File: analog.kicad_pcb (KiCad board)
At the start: 2 copper layers, 80 x 40 mm, 65 parts, among them P1 CONN_01X09, P2 CONN_01X06, P3 CONN_01X06, P4 CONN_01X05, U1 LM2940, U2 TLC2543

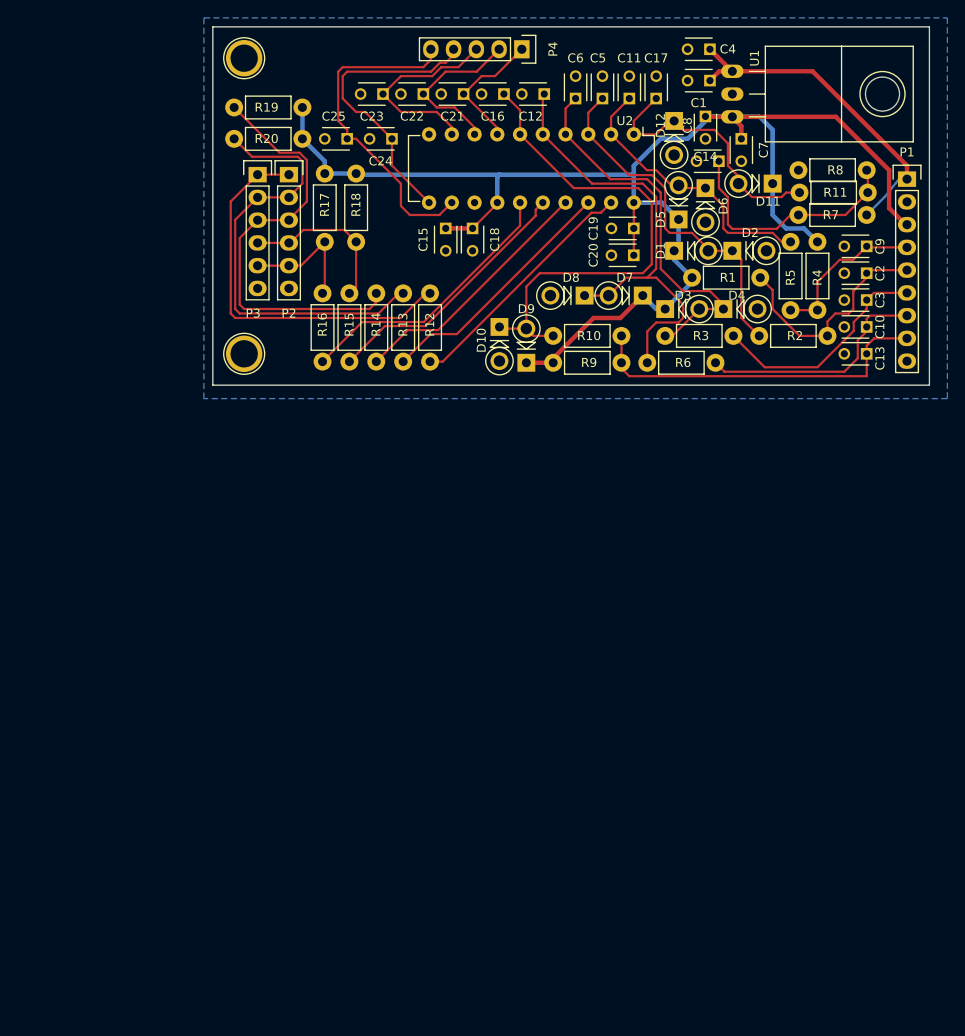
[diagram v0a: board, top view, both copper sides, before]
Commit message: fixups
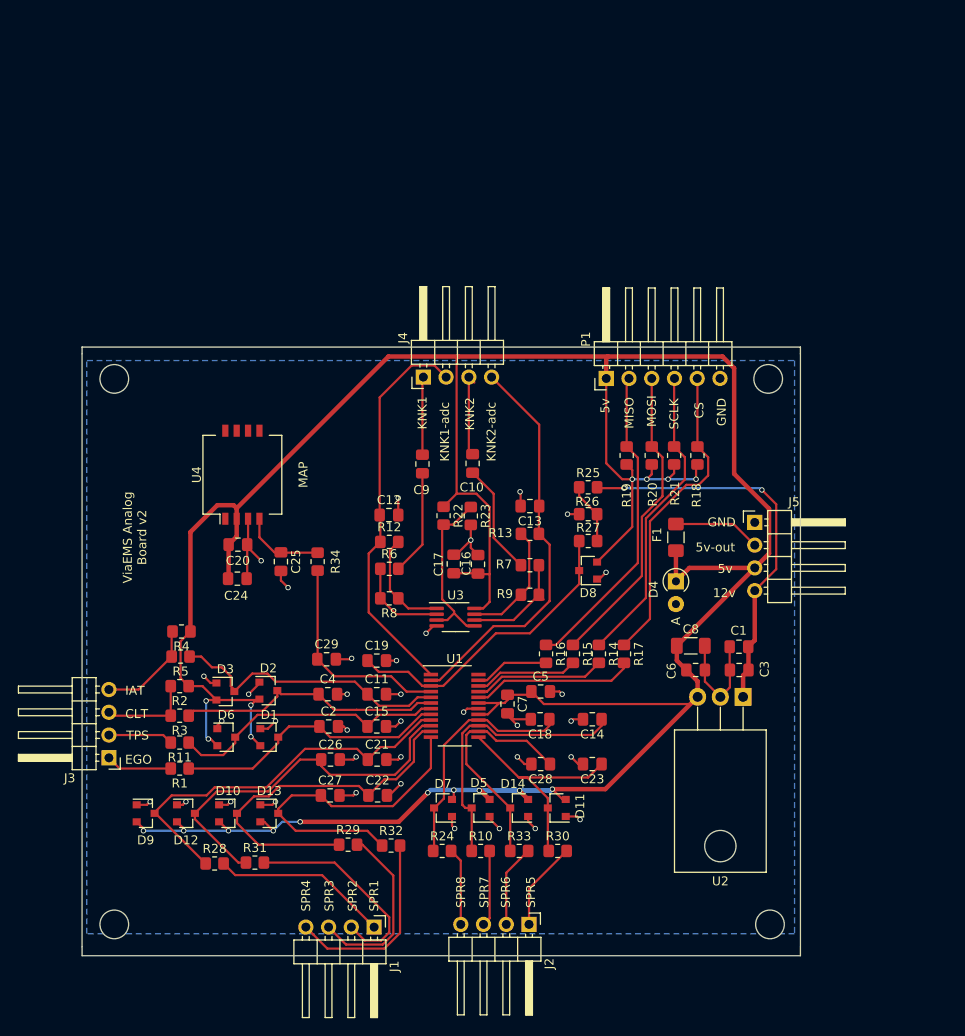
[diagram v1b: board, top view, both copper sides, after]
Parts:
- removed ?: 1pin, Connect:1pin
- removed P2, P3: CONN_01X06, Pin_Headers:Pin_Header_Straight_1x06
- removed P4: CONN_01X05, Pin_Headers:Pin_Header_Straight_1x05
- removed the REF** at (48.5, 69.0)
- added C26: 0.47 uF, Capacitor_SMD:C_0805_2012Metric_Pad1.18x1.45mm_HandSolder, F.Cu at (58.1, 147.3)
- added C27: 0.47 uF, Capacitor_SMD:C_0805_2012Metric_Pad1.18x1.45mm_HandSolder, F.Cu at (58.1, 151.3)
- added C28: 0.47 uF, Capacitor_SMD:C_0805_2012Metric_Pad1.18x1.45mm_HandSolder, F.Cu at (81.6, 147.8)
- added C29: 0.47 uF, Capacitor_SMD:C_0805_2012Metric_Pad1.18x1.45mm_HandSolder, F.Cu at (57.7, 136.1)
- added D13: BAT54S, Package_TO_SOT_SMD:SOT-23, F.Cu at (51.3, 153.3)
- added D14: BAT54S, Package_TO_SOT_SMD:SOT-23, F.Cu at (79.2, 152.7)
- added F1: 500 mA, Fuse:Fuse_1206_3216Metric_Pad1.42x1.75mm_HandSolder, F.Cu at (96.7, 122.5)
- added J1: SPARE1, Connector_PinHeader_2.54mm:PinHeader_1x04_P2.54mm_Horizontal, F.Cu at (63.0, 166.0)
- added J2: SPARE2, Connector_PinHeader_2.54mm:PinHeader_1x04_P2.54mm_Horizontal, F.Cu at (80.3, 165.7)
- added J3: MAIN, Connector_PinHeader_2.54mm:PinHeader_1x04_P2.54mm_Horizontal, F.Cu at (33.4, 147.1)
- added J4: KNOCK, Connector_PinHeader_2.54mm:PinHeader_1x04_P2.54mm_Horizontal, F.Cu at (68.5, 104.6)
- added J5: POWER, Connector_PinHeader_2.54mm:PinHeader_1x04_P2.54mm_Horizontal, F.Cu at (105.5, 120.8)
- added R21: 10k, Resistor_SMD:R_0805_2012Metric_Pad1.20x1.40mm_HandSolder, F.Cu at (96.5, 113.3)
- added R22: 1000, Resistor_SMD:R_0805_2012Metric_Pad1.20x1.40mm_HandSolder, F.Cu at (70.8, 120.1)
- added R23: 1000, Resistor_SMD:R_0805_2012Metric_Pad1.20x1.40mm_HandSolder, F.Cu at (73.8, 120.1)
- added R24: 220, Resistor_SMD:R_0805_2012Metric_Pad1.20x1.40mm_HandSolder, F.Cu at (70.6, 157.5)
- added R25: 3.9k, Resistor_SMD:R_0805_2012Metric_Pad1.20x1.40mm_HandSolder, F.Cu at (86.9, 116.9)
- added R26: 1k, Resistor_SMD:R_0805_2012Metric_Pad1.20x1.40mm_HandSolder, F.Cu at (86.9, 119.9)
- added R27: 220, Resistor_SMD:R_0805_2012Metric_Pad1.20x1.40mm_HandSolder, F.Cu at (86.9, 122.9)
- added R28: 220, Resistor_SMD:R_0805_2012Metric_Pad1.20x1.40mm_HandSolder, F.Cu at (45.2, 158.9)
- added R29: 220, Resistor_SMD:R_0805_2012Metric_Pad1.20x1.40mm_HandSolder, F.Cu at (60.1, 156.8)
- added R30: 220, Resistor_SMD:R_0805_2012Metric_Pad1.20x1.40mm_HandSolder, F.Cu at (83.5, 157.5)
- added R31: 220, Resistor_SMD:R_0805_2012Metric_Pad1.20x1.40mm_HandSolder, F.Cu at (49.7, 158.8)
- added R32: 220, Resistor_SMD:R_0805_2012Metric_Pad1.20x1.40mm_HandSolder, F.Cu at (64.9, 156.9)
- added R33: 220, Resistor_SMD:R_0805_2012Metric_Pad1.20x1.40mm_HandSolder, F.Cu at (79.2, 157.5)
- added R34: 220, Resistor_SMD:R_0805_2012Metric_Pad1.20x1.40mm_HandSolder, F.Cu at (56.7, 125.2)
- added REF**: MountingHole_3.2mm_M3, MountingHole:MountingHole_3.2mm_M3, F.Cu at (34.0, 165.7)
- added REF**: MountingHole_3.2mm_M3, MountingHole:MountingHole_3.2mm_M3, F.Cu at (107.2, 165.7)
- added REF**: MountingHole_3.2mm_M3, MountingHole:MountingHole_3.2mm_M3, F.Cu at (107.0, 104.8)
- added REF**: MountingHole_3.2mm_M3, MountingHole:MountingHole_3.2mm_M3, F.Cu at (34.0, 104.8)
- added U3: MCP6002-xSN, Package_SO:MSOP-8_3x3mm_P0.65mm, F.Cu at (72.1, 131.4)
- added U4: MPXA6400A, Sensor_Pressure:Freescale_98ARH99089A, F.Cu at (48.3, 115.5)
- C1, C10, C13, C21, C22, C23, C3, C7, C9: footprint Capacitors_ThroughHole:C_Disc_D3_P2.5 -> Capacitor_SMD:C_0805_2012Metric_Pad1.18x1.45mm_HandSolder
- C11, C16: value 0.47 uF -> 1 uF; footprint Capacitors_ThroughHole:C_Disc_D3_P2.5 -> Capacitor_SMD:C_0805_2012Metric_Pad1.18x1.45mm_HandSolder
- C12, C17, C25, C5, C6: value 0.47 uF -> 0.1 uF; footprint Capacitors_ThroughHole:C_Disc_D3_P2.5 -> Capacitor_SMD:C_0805_2012Metric_Pad1.18x1.45mm_HandSolder
- C14, C2: value 0.1 uF -> 0.47 uF; footprint Capacitors_ThroughHole:C_Disc_D3_P2.5 -> Capacitor_SMD:C_0805_2012Metric_Pad1.18x1.45mm_HandSolder
- C15, C19, C4: value 0.1 uF -> 1 uF; footprint Capacitors_ThroughHole:C_Disc_D3_P2.5 -> Capacitor_SMD:C_0805_2012Metric_Pad1.18x1.45mm_HandSolder
- C18: value 10 uF -> 0.47 uF; footprint Capacitors_ThroughHole:C_Disc_D3_P2.5 -> Capacitor_SMD:C_0805_2012Metric_Pad1.18x1.45mm_HandSolder
- C20: value 10 uF -> 0.01 uF; footprint Capacitors_ThroughHole:C_Disc_D3_P2.5 -> Capacitor_SMD:C_0805_2012Metric_Pad1.18x1.45mm_HandSolder
- C24: value 0.47 uF -> 0.33 uF; footprint Capacitors_ThroughHole:C_Disc_D3_P2.5 -> Capacitor_SMD:C_0805_2012Metric_Pad1.18x1.45mm_HandSolder
- C8: footprint Capacitors_ThroughHole:C_Disc_D3_P2.5 -> Capacitor_SMD:C_1206_3216Metric_Pad1.33x1.80mm_HandSolder
- D1, D10, D11, D12, D2, D3, D5, D6, D7, D8, D9: value 1N5818 -> BAT54S; footprint Diodes_ThroughHole:Diode_DO-41_SOD81_Vertical_KathodeUp -> Package_TO_SOT_SMD:SOT-23
- D4: value 1N5818 -> 5.4 V; footprint Diodes_ThroughHole:Diode_DO-41_SOD81_Vertical_KathodeUp -> Diode_THT:D_A-405_P2.54mm_Vertical_AnodeUp
- P1: value CONN_01X09 -> CONN_01X06; footprint Pin_Headers:Pin_Header_Straight_1x09 -> Connector_PinHeader_2.54mm:PinHeader_1x06_P2.54mm_Horizontal
- R1: value 2.49k -> 220; footprint Resistors_ThroughHole:Resistor_Horizontal_RM7mm -> Resistor_SMD:R_0805_2012Metric_Pad1.20x1.40mm_HandSolder
- R10, R11, R3, R5: value 470 -> 220; footprint Resistors_ThroughHole:Resistor_Horizontal_RM7mm -> Resistor_SMD:R_0805_2012Metric_Pad1.20x1.40mm_HandSolder
- R12, R13: value 100 -> 120; footprint Resistors_ThroughHole:Resistor_Horizontal_RM7mm -> Resistor_SMD:R_0805_2012Metric_Pad1.20x1.40mm_HandSolder
- R14, R15, R16, R18, R19, R20, R4: footprint Resistors_ThroughHole:Resistor_Horizontal_RM7mm -> Resistor_SMD:R_0805_2012Metric_Pad1.20x1.40mm_HandSolder
- R17: value 10k -> 100; footprint Resistors_ThroughHole:Resistor_Horizontal_RM7mm -> Resistor_SMD:R_0805_2012Metric_Pad1.20x1.40mm_HandSolder
- R2: value 470 -> 2.49k; footprint Resistors_ThroughHole:Resistor_Horizontal_RM7mm -> Resistor_SMD:R_0805_2012Metric_Pad1.20x1.40mm_HandSolder
- R6: value 470 -> 1000; footprint Resistors_ThroughHole:Resistor_Horizontal_RM7mm -> Resistor_SMD:R_0805_2012Metric_Pad1.20x1.40mm_HandSolder
- R7: value 3.9k -> 1000; footprint Resistors_ThroughHole:Resistor_Horizontal_RM7mm -> Resistor_SMD:R_0805_2012Metric_Pad1.20x1.40mm_HandSolder
- R8: value 1k -> 330; footprint Resistors_ThroughHole:Resistor_Horizontal_RM7mm -> Resistor_SMD:R_0805_2012Metric_Pad1.20x1.40mm_HandSolder
- R9: value 2.49k -> 330; footprint Resistors_ThroughHole:Resistor_Horizontal_RM7mm -> Resistor_SMD:R_0805_2012Metric_Pad1.20x1.40mm_HandSolder
- U1: value LM2940 -> MAX11632; footprint TO_SOT_Packages_THT:TO-220_Neutral123_Horizontal -> Package_SO:QSOP-24_3.9x8.7mm_P0.635mm
- U2: value TLC2543 -> LM2940; footprint Housings_DIP:DIP-20_W7.62mm -> Package_TO_SOT_THT:TO-220-3_Horizontal_TabDown
- moved D12 94.6 mm to (42.0, 153.3), turned to 0 degrees
- moved R11 92.5 mm to (41.3, 145.4), turned to 180 degrees
- moved C4 83.7 mm to (57.8, 140.0), turned to 0 degrees
- moved R4 83.3 mm to (41.5, 133.0), turned to 180 degrees
- moved R5 82.3 mm to (41.4, 135.8), turned to 180 degrees
- moved D6 81.4 mm to (46.5, 144.8), turned to 0 degrees
- moved R1 79.2 mm to (41.3, 148.3), turned to 180 degrees
- moved C2 78.5 mm to (57.9, 143.6), turned to 0 degrees
- moved C22 78.5 mm to (63.4, 151.3), turned to 0 degrees
- moved C23 78.4 mm to (87.4, 147.8)
- moved R2 75.6 mm to (41.3, 139.1), turned to 180 degrees
- moved U1 75.0 mm to (72.0, 141.3), turned to 0 degrees
- moved C21 74.9 mm to (63.3, 147.3), turned to 0 degrees
- moved D11 73.7 mm to (83.4, 152.7)
- moved C11 72.2 mm to (63.3, 140.0), turned to 0 degrees
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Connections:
- C10 pad 1: EGO-in -> Net-(C10-Pad1)
- C10 pad 2: GND -> KNK2
- C12 pad 1: EGO-adc -> KNK1-adc
- C13 pad 1: SPR-in -> KNK2-adc
- C14 pad 1: Net-(C14-Pad1) -> SPR7-adc
- C15 pad 1: 5v_analog -> TPS-adc
- C16 pad 1: SPR-adc -> 5v_analog
- C17 pad 1: BRV-adc -> 5v_analog
- C18 pad 1: 5v_analog -> SPR8-adc
- C19 pad 1: 5v_analog -> BRV-adc
- C2 pad 1: CLT-in -> EGO-adc
- C21 pad 1: EX-1 -> SPR1-adc
- C22 pad 1: EX-2 -> SPR3-adc
- C23 pad 1: EX-3 -> SPR5-adc
- C24 pad 1: EX-4 -> 5v_analog
- C25 pad 1: EX-5 -> Net-(C25-Pad1)
- C3 pad 1: TPS-in -> 12v_analog
- C4 pad 1: 12v_analog -> CLT-adc
- C5 pad 1: CLT-adc -> 5v_analog
- C6 pad 1: TPS-adc -> 5v_analog
- C9 pad 1: IAT-in -> Net-(C9-Pad1)
- C9 pad 2: GND -> KNK1
- D1 pad 1: 5v_analog -> GND
- D1 pad 2: CLT-adc -> 5v_analog
- D10 pad 1: SPR-adc -> GND
- D10 pad 2: GND -> 5v_analog
- D11 pad 1: 5v_analog -> GND
- D11 pad 2: BRV-adc -> 5v_analog
- D12 pad 1: BRV-adc -> GND
- D12 pad 2: GND -> 5v_analog
- D2 pad 1: CLT-adc -> GND
- D2 pad 2: GND -> 5v_analog
- D3 pad 1: 5v_analog -> GND
- D3 pad 2: TPS-adc -> 5v_analog
- D4 pad 1: TPS-adc -> 5v_analog
- D5 pad 1: 5v_analog -> GND
- D5 pad 2: IAT-adc -> 5v_analog
- D6 pad 1: IAT-adc -> GND
- D6 pad 2: GND -> 5v_analog
- D7 pad 1: 5v_analog -> GND
- D7 pad 2: EGO-adc -> 5v_analog
- D8 pad 1: EGO-adc -> GND
- D8 pad 2: GND -> 5v_analog
- D9 pad 1: 5v_analog -> GND
- D9 pad 2: SPR-adc -> 5v_analog
- P1 pad 1: 12v_analog -> 5v_analog
- P1 pad 2: GND -> Net-(P1-Pad2)
- P1 pad 3: 5v_analog -> Net-(P1-Pad3)
- P1 pad 4: IAT-in -> Net-(P1-Pad4)
- P1 pad 5: CLT-in -> Net-(P1-Pad5)
- P1 pad 6: TPS-in -> GND
- R1 pad 1: 5v_analog -> EGO-adc
- R1 pad 2: CLT-in -> EGO-in
- R10 pad 1: SPR-adc -> SPR7-adc
- R10 pad 2: SPR-in -> SPR7-in
- R11 pad 1: BRV-adc -> TPS-adc
- R11 pad 2: Net-(C14-Pad1) -> TPS-in
- R12 pad 1: Net-(P2-Pad1) -> KNK1-adc
- R12 pad 2: ADC_EOC -> Net-(R12-Pad2)
- R13 pad 1: Net-(P2-Pad2) -> KNK2-adc
- R13 pad 2: ADC_CLK -> Net-(R13-Pad2)
- R14 pad 1: Net-(P2-Pad3) -> Net-(P1-Pad4)
- R14 pad 2: ADC_MOSI -> ADC_CLK
- R15 pad 1: Net-(P2-Pad4) -> Net-(P1-Pad3)
- R15 pad 2: ADC_MISO -> ADC_MOSI
- R16 pad 1: Net-(P2-Pad5) -> Net-(P1-Pad2)
- R16 pad 2: ADC_CS -> ADC_MISO
- R17 pad 1: 5v_analog -> Net-(P1-Pad5)
- R17 pad 2: Net-(P2-Pad5) -> ADC_CS
- R18 pad 2: Net-(P2-Pad4) -> Net-(P1-Pad5)
- R19 pad 2: Net-(P2-Pad3) -> Net-(P1-Pad2)
- R2 pad 1: CLT-adc -> 5v_analog
- R20 pad 2: Net-(P2-Pad2) -> Net-(P1-Pad3)
- R3 pad 1: TPS-adc -> CLT-adc
- R3 pad 2: TPS-in -> CLT-in
- R6 pad 1: EGO-adc -> Net-(R6-Pad1)
- R6 pad 2: EGO-in -> Net-(C9-Pad1)
- R7 pad 1: 12v_analog -> Net-(R7-Pad1)
- R7 pad 2: Net-(C14-Pad1) -> Net-(C10-Pad1)
- R8 pad 1: Net-(C14-Pad1) -> Net-(R12-Pad2)
- R8 pad 2: GND -> Net-(R6-Pad1)
- R9 pad 1: 5v_analog -> Net-(R13-Pad2)
- R9 pad 2: SPR-in -> Net-(R7-Pad1)
- U1 pad 1: 12v_analog -> KNK1-adc
- U1 pad 2: GND -> KNK2-adc
- U1 pad 3: 5v_analog -> BRV-adc
- U2 pad 1: BRV-adc -> 12v_analog
- U2 pad 2: IAT-adc -> GND
- U2 pad 3: CLT-adc -> 5v_analog
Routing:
- net 5v_analog: track 171.7 -> 362.9 mm, vias 0 -> 18
- net GND: track 0.00 -> 86.9 mm, vias 0 -> 36
- net SPR-adc: track 56.2 -> 0.00 mm
- net Net-(P2-Pad2): track 50.2 -> 0.00 mm
- net Net-(P2-Pad3): track 48.6 -> 0.00 mm
- net KNK2-adc: track 0.00 -> 44.6 mm
- net SPR1-adc: track 0.00 -> 44.2 mm
- net Net-(P2-Pad1): track 43.8 -> 0.00 mm
- net KNK1-adc: track 0.00 -> 43.8 mm
- net SPR2-adc: track 0.00 -> 42.0 mm
- net SPR3-adc: track 0.00 -> 41.2 mm
- net SPR-in: track 39.6 -> 0.00 mm
- net EX-5: track 37.2 -> 0.00 mm
- net SPR4-adc: track 0.00 -> 37.0 mm
- net Net-(P1-Pad2): track 0.00 -> 35.3 mm
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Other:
- board size 80 x 40 mm -> 80.2 x 67.9 mm
- board text added: "12v"
- board text added: "5v"
- board text added: "5v-out"
- board text added: "CLT"
- board text added: "CS"
- board text added: "EGO"
- board text added: "GND"
- board text added: "IAT"
- board text added: "KNK1"
- board text added: "KNK1-adc"
- board text added: "KNK2"
- board text added: "KNK2-adc"
- board text added: "MAP"
- board text added: "MISO"
- board text added: "MOSI"
- board text added: "SCLK"
- board text added: "SPR1"
- board text added: "SPR2"
- board text added: "SPR3"
- board text added: "SPR4"
- board text added: "SPR5"
- board text added: "SPR6"
- board text added: "SPR7"
- board text added: "SPR8"
- board text added: "TPS"
- board text added: "ViaEMS Analog Board v2"
